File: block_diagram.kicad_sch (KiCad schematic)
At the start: 0 parts

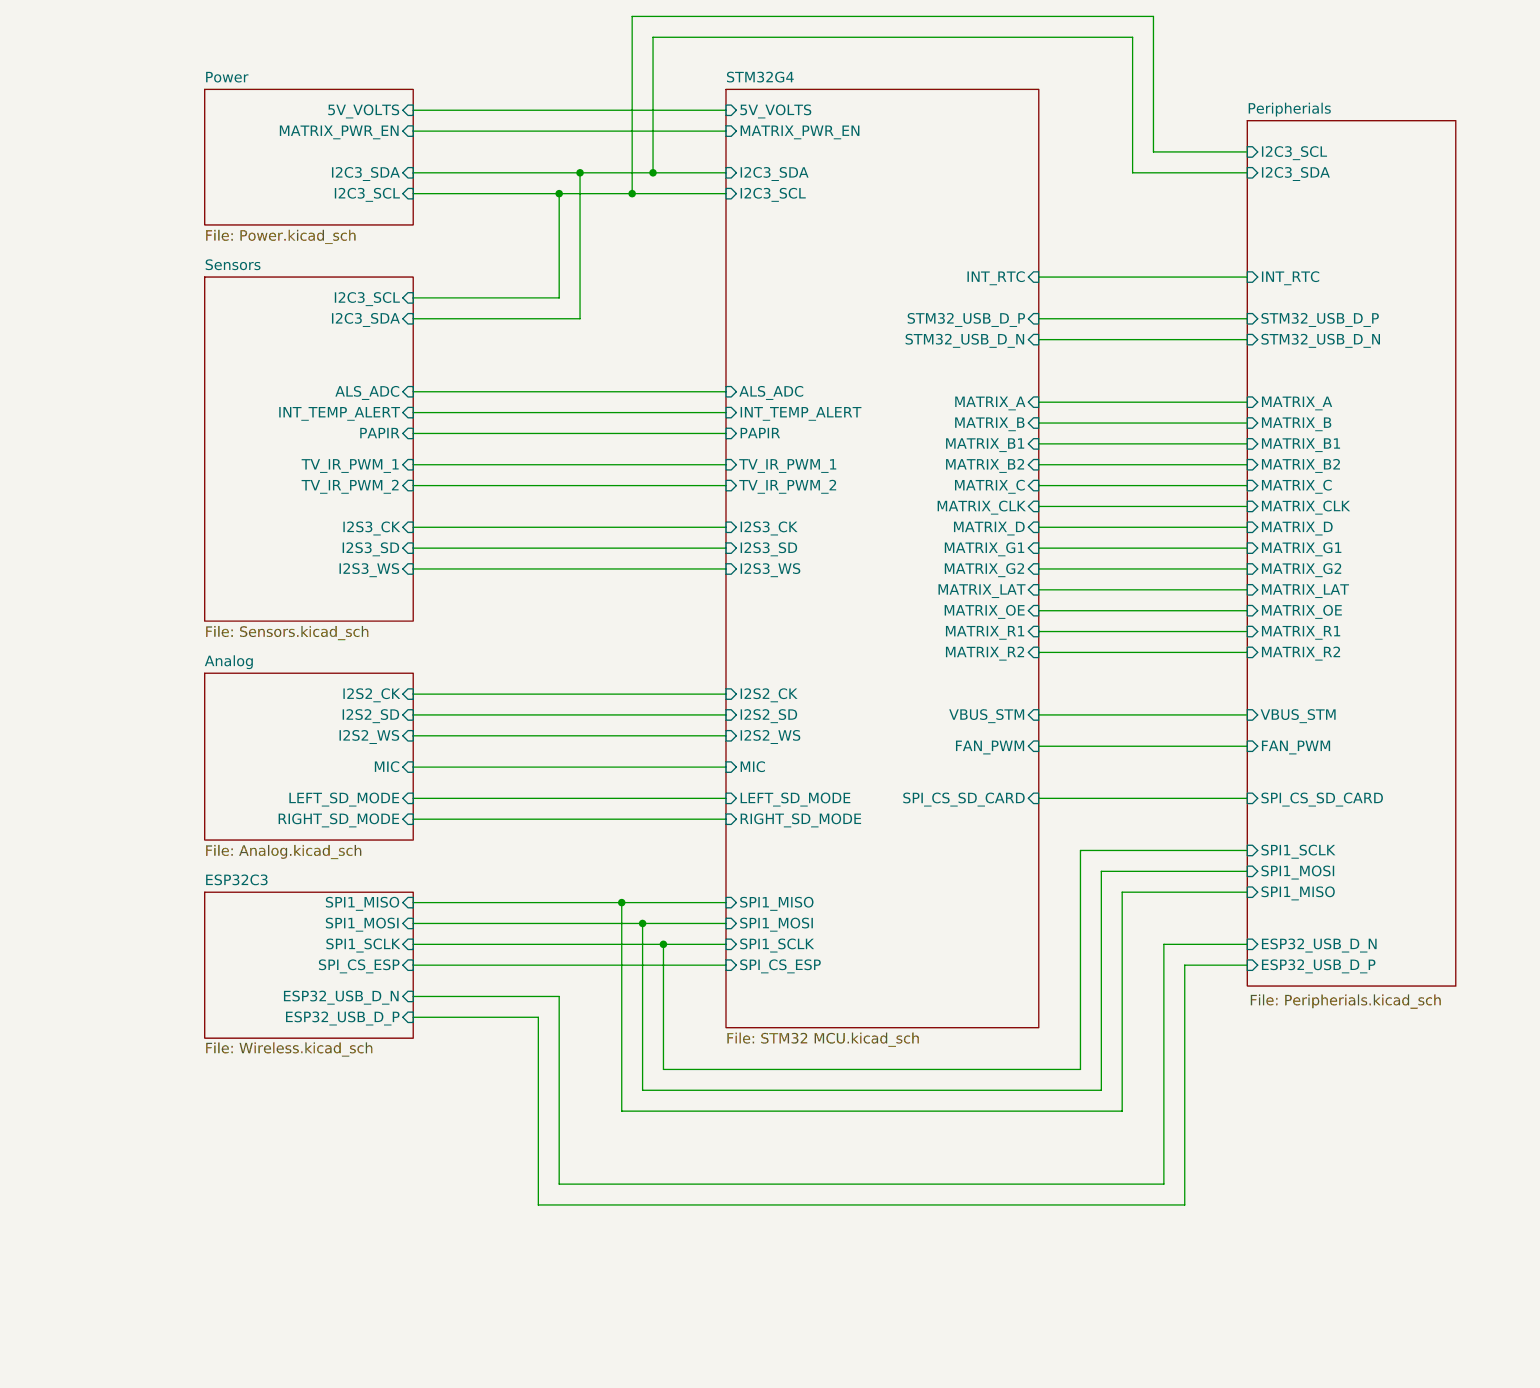
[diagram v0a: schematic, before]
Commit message: working on power delivery
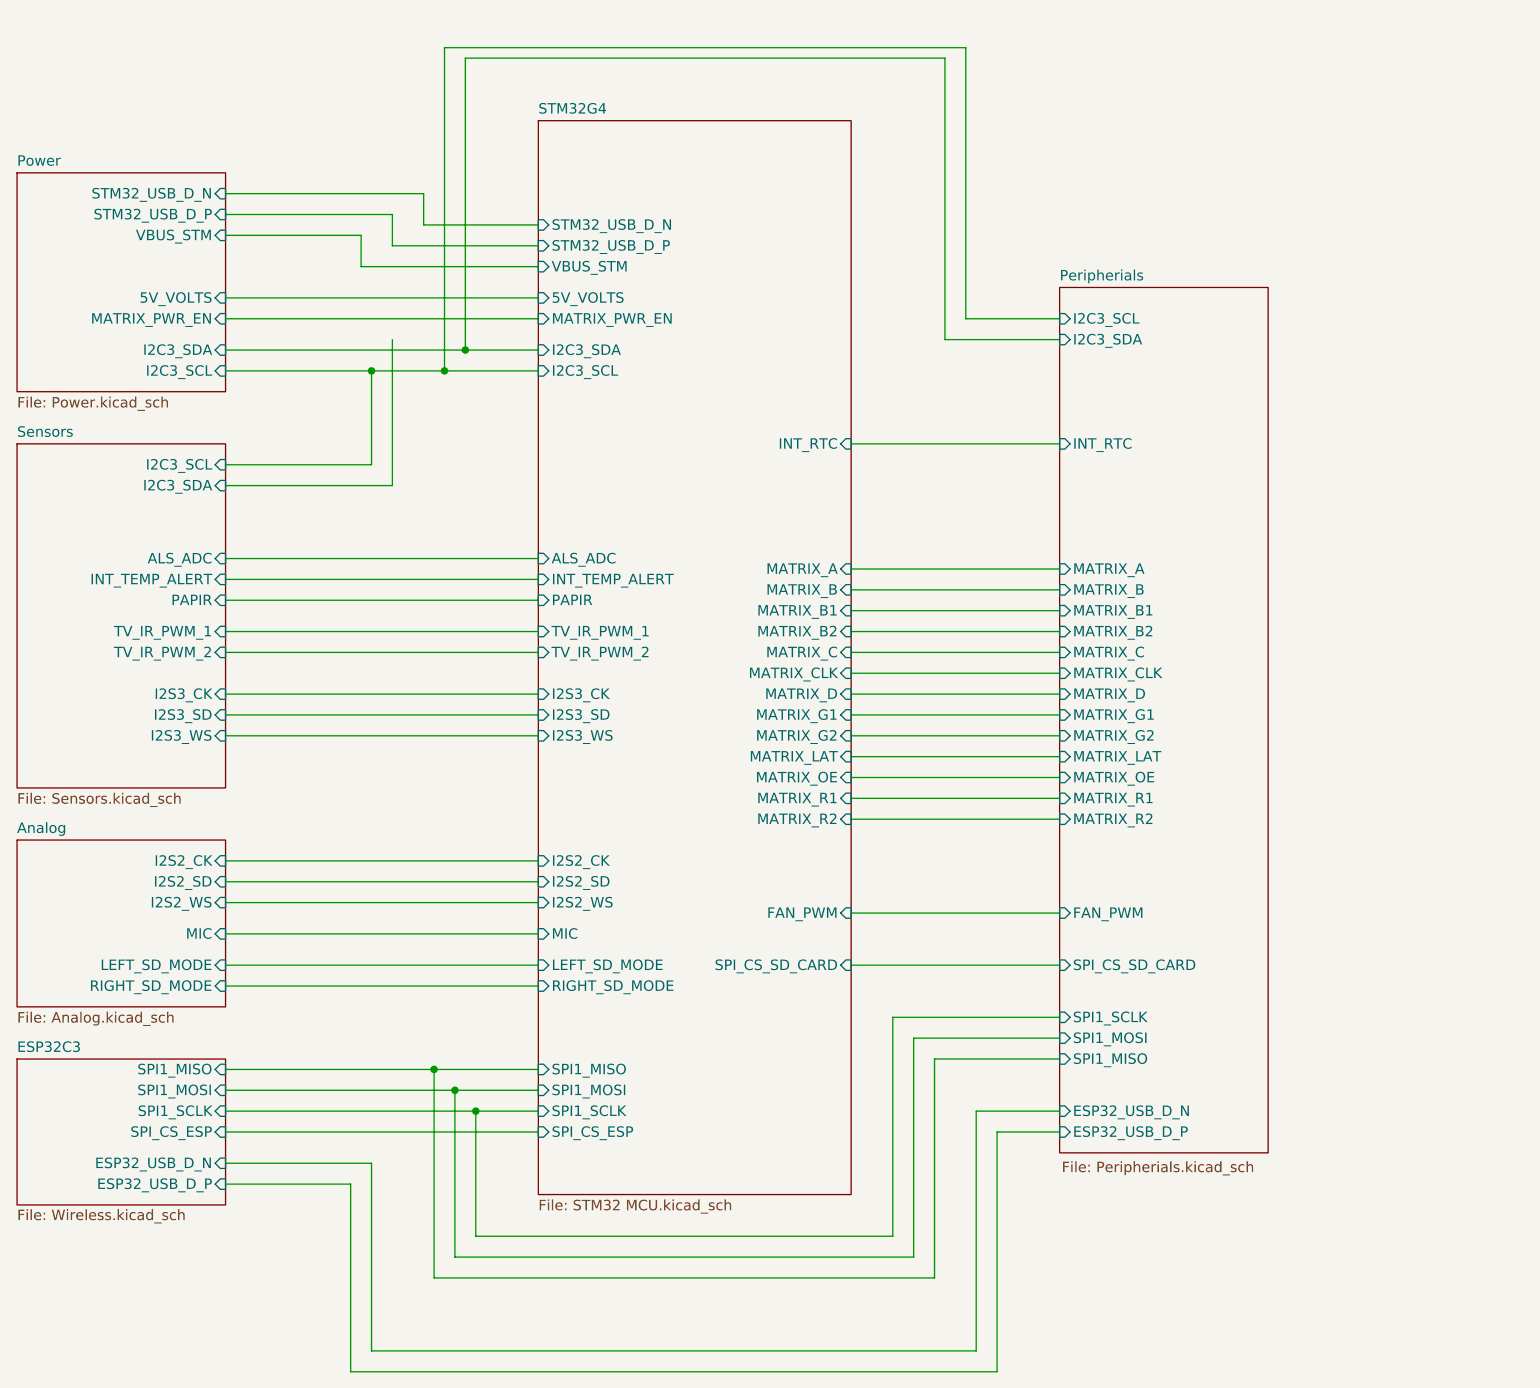
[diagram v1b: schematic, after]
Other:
- sheet Peripherials ports: added none; removed STM32_USB_D_N, STM32_USB_D_P, VBUS_STM
- sheet Power ports: added STM32_USB_D_N, STM32_USB_D_P, VBUS_STM; removed none
